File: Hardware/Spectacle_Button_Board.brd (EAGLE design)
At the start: 44.5 x 73.7 mm, 50 parts, among them J17 AUDIO-JACK3, J19 FTDI_DEVICE, J20 AUDIO-JACK3, U1 CY8C4146LQI-S422, U2 3.3V/150mA

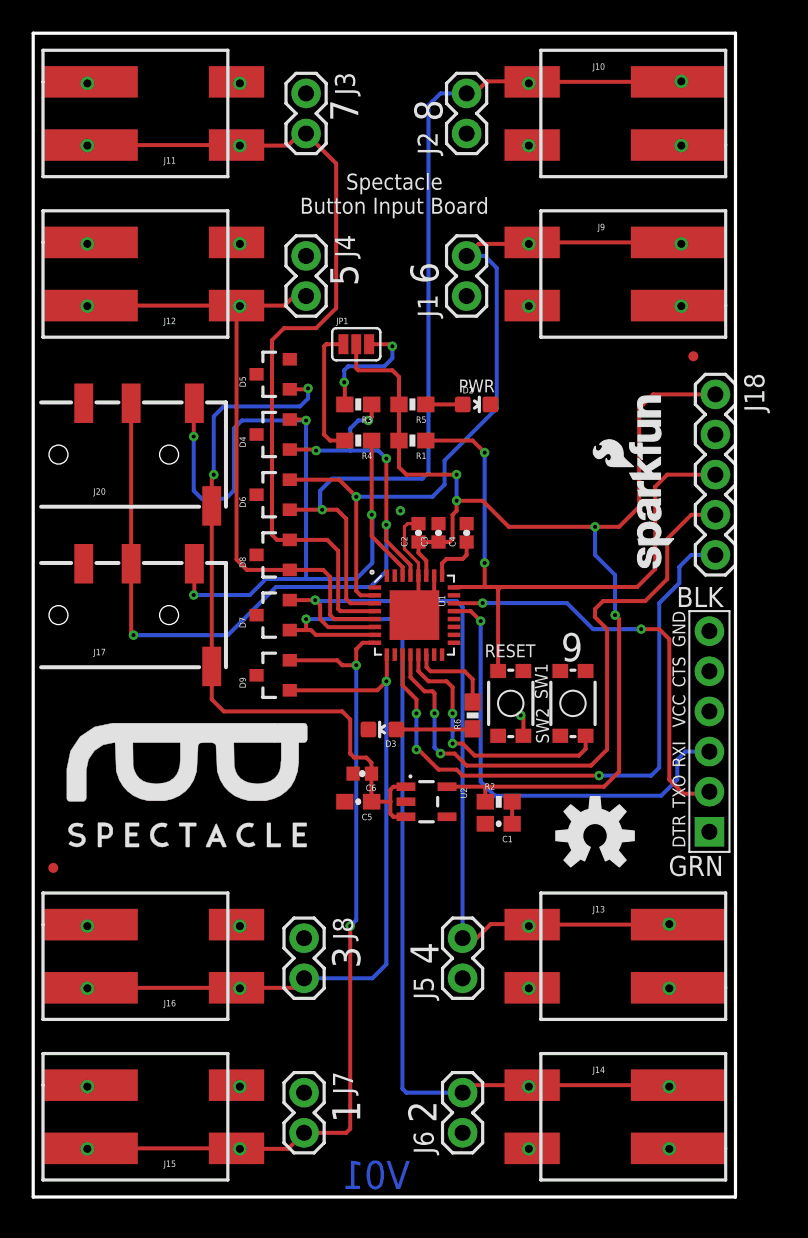
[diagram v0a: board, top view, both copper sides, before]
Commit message: Quick schematic changes, ready for QC review
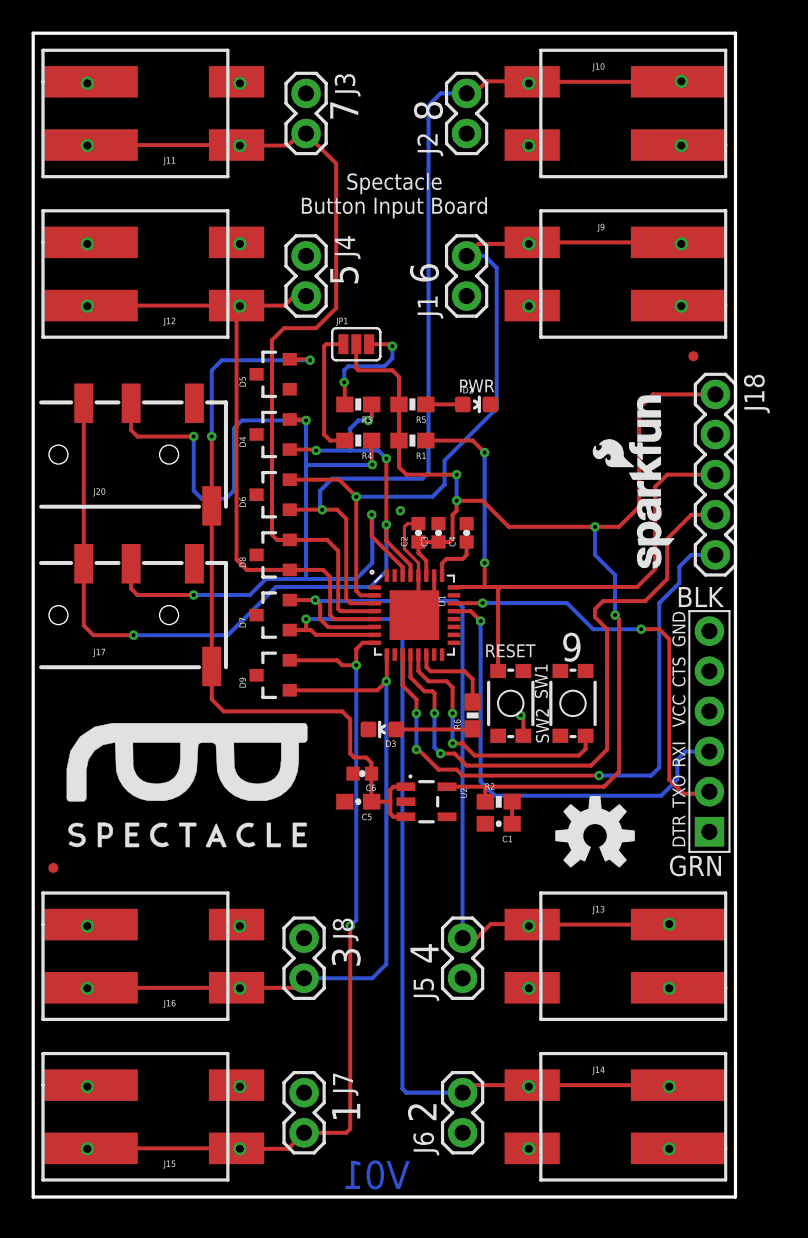
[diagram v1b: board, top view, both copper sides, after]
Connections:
- net GND: now also J17.TIP, J20.TIP; no longer J17.RING2, J20.RING2
- net SCL: now also J17.RING2, J20.RING2; no longer J17.RING1, J20.RING1
- net SDA: now also J17.RING1, J20.RING1; no longer J17.TIP, J20.TIP
- net VIN: now also D5.2; no longer D5.1
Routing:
- net SDA: track 54.9 -> 63.4 mm, vias 4 -> 5
- net SCL: track 53.6 -> 56.3 mm
- net VIN: track 46.6 -> 49.0 mm
- net IN_6: track 53.2 -> 54.9 mm
